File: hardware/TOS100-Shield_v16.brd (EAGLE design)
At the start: 68.6 x 53.3 mm, 65 parts, among them IC1 TMC260-PA, J1 POWER_JACKPTH, T1 N-Chn, T2 N-Chn, T3 P-Chn, T4 N-Chn

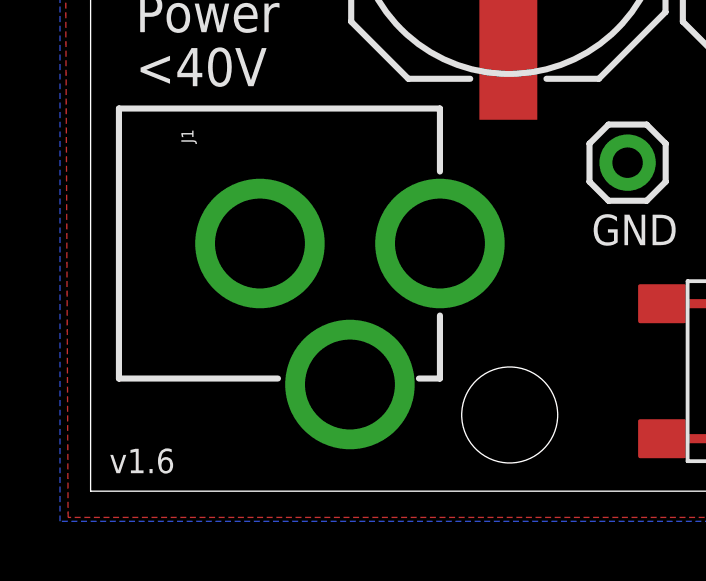
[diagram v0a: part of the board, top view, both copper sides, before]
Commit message: updated layout and schematics
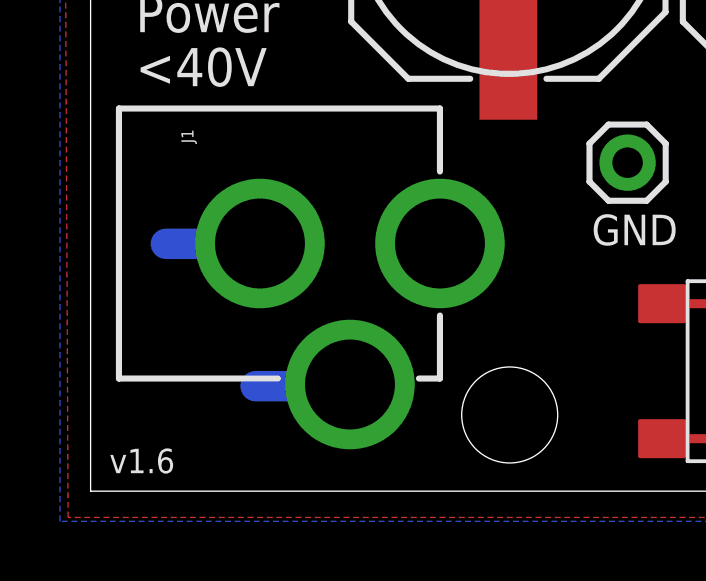
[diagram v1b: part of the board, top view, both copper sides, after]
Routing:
- net GND: track 55.6 -> 61.8 mm
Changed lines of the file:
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@@
 <board>
 <plain>
-<circle x="66" y="35.625" radius="3.1349" width="0.8128" layer="41"/>
 <circle x="14" y="2.5" radius="3.2" width="0" layer="41"/>
-<circle x="65.75" y="35.625" radius="3.1349" width="0.8128" layer="42"/>
-<circle x="15.125" y="50.75" radius="3.1349" width="0.8128" layer="42"/>
-<circle x="14.375" y="2.625" radius="3.2" width="0" layer="42"/>
+<circle x="14" y="2.5" radius="3.2" width="0" layer="42"/>
 <text x="54.875" y="26.375" size="1.016" layer="25" rot="R90">A1</text>
 <text x="54.875" y="24" size="1.016" layer="25" rot="R90">A2</text>
@@
 <text x="0" y="-2" size="1.27" layer="49" font="vector" ratio="10" align="top-left">Silkscreen: 21 tPlace + 25 tNames</text>
 <circle x="47.6325" y="36.3025" radius="0.1" width="0.25" layer="21"/>
+<circle x="66" y="35.5" radius="3.5" width="0" layer="42"/>
+<circle x="66" y="35.5" radius="3.5" width="0" layer="41"/>
+<circle x="15.125" y="50.75" radius="3.5" width="0" layer="41"/>
+<circle x="15.125" y="50.75" radius="3.5" width="0" layer="42"/>
 </plain>
 <attributes>
@@
 <wire x1="35.2" y1="29.4" x2="34.94" y2="29.4" width="0.4064" layer="1"/>
 <wire x1="34.94" y1="29.4" x2="34.895" y2="29.445" width="0.4064" layer="1"/>
+<wire x1="2.51" y1="8.245" x2="5.705" y2="8.245" width="1.016" layer="16"/>
+<wire x1="5.5" y1="3.5" x2="8.5" y2="3.5" width="1.016" layer="16"/>
 </signal>
 <signal name="3V">
